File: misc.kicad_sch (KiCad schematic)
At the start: 62 parts, among them J1 Serial 1, J10 SW2, J11 SW2, J12 SW2, J13 Rotary Encoder, J14 Paddles, J15 Conn_02x07_Row_Letter_Last, J17 Conn_02x04_Row_Letter_Last, J18 Conn_02x04_Top_Bottom, J19 I2C, J21 Serial 2, J22 Rotary Encoder, J3 Serial 2, J4 KeyerOut1, J5 KeyerOut2, J6 SW2, J7 SW2, J8 SW2, J9 SW2, Q1 2N7000, Q2 2N7000, Q3 2N7000, Q4 2N7000, U1 LCD 16x2 16x4 20x4

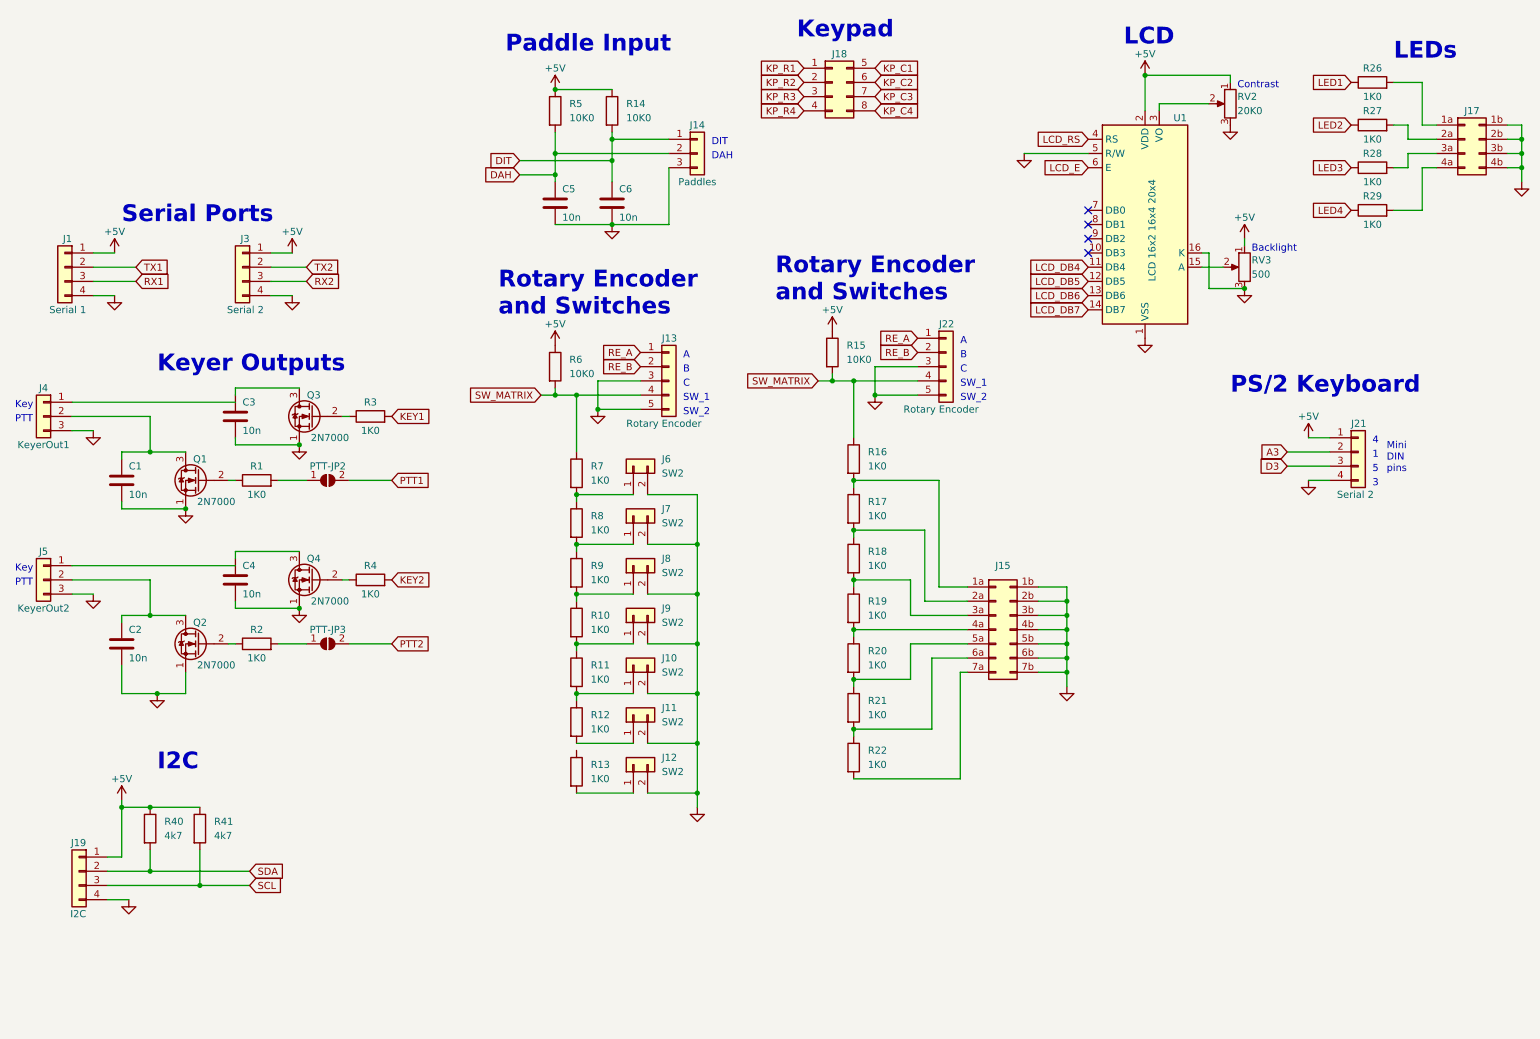
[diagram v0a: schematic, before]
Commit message: Small drawing cleanups.
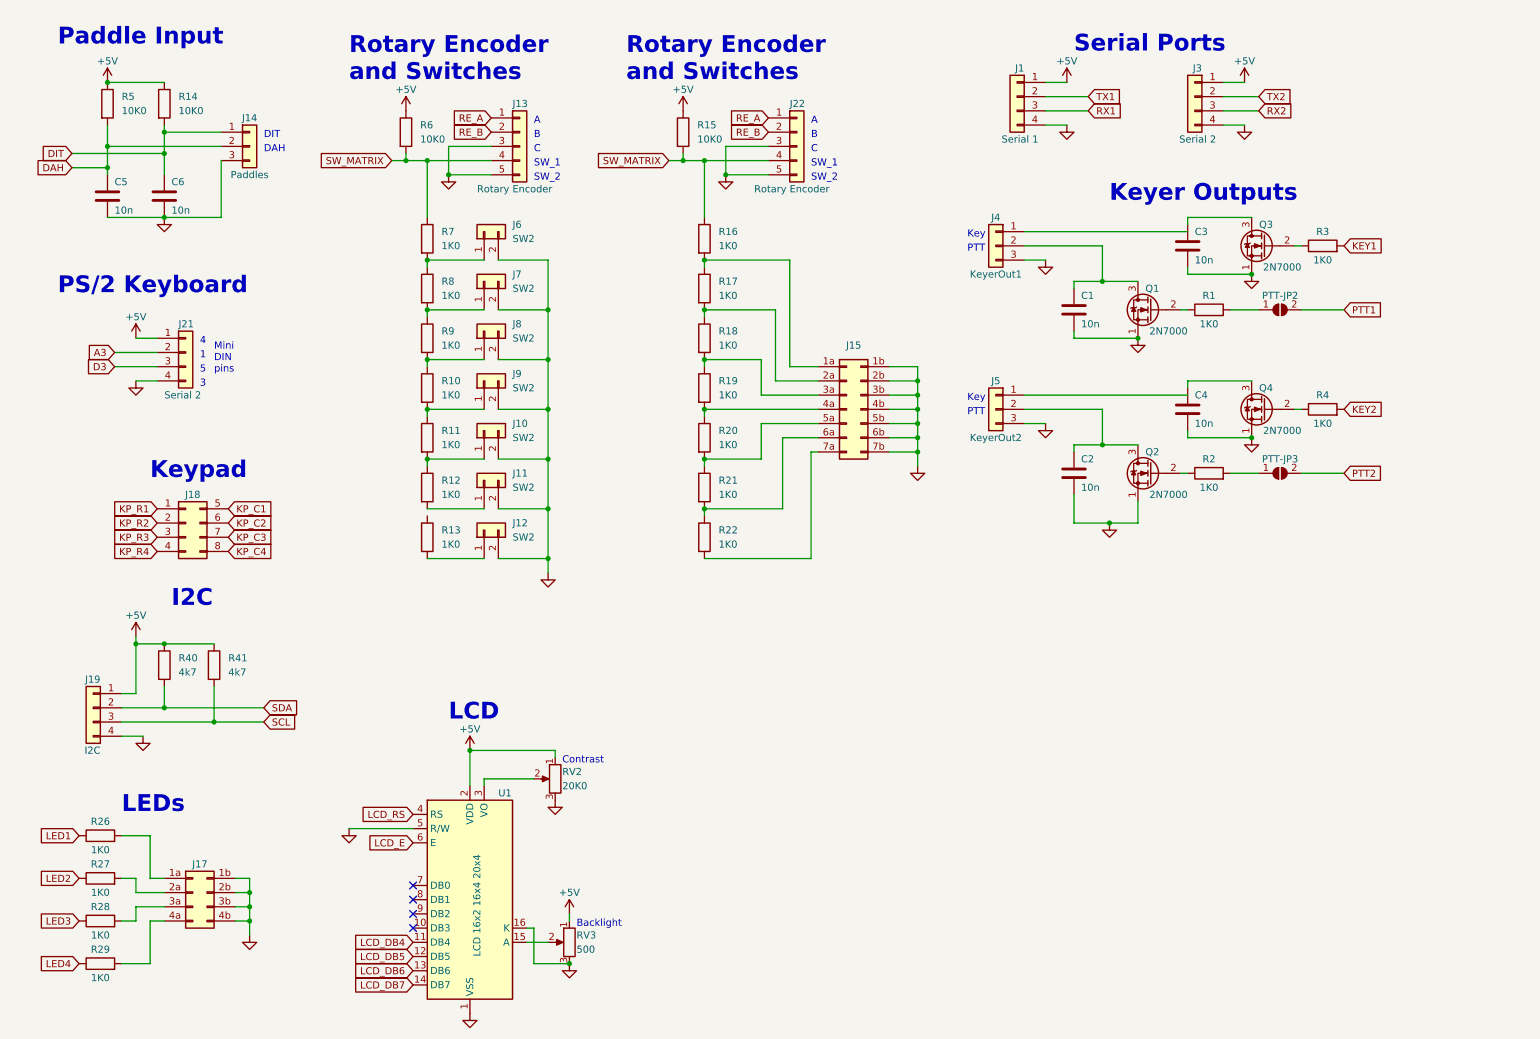
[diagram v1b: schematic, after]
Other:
- company: (none) -> EZ Electronics
- title: (none) -> Arduino Mega2560 K3NG Keyer - Miscellaneous Circuits
- moved on the sheet: C1, C2, C3, C4, C5, C6, J1, J10, J11, J12, J13, J14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
